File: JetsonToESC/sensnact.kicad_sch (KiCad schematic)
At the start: 8 parts, among them U2 DS18B20

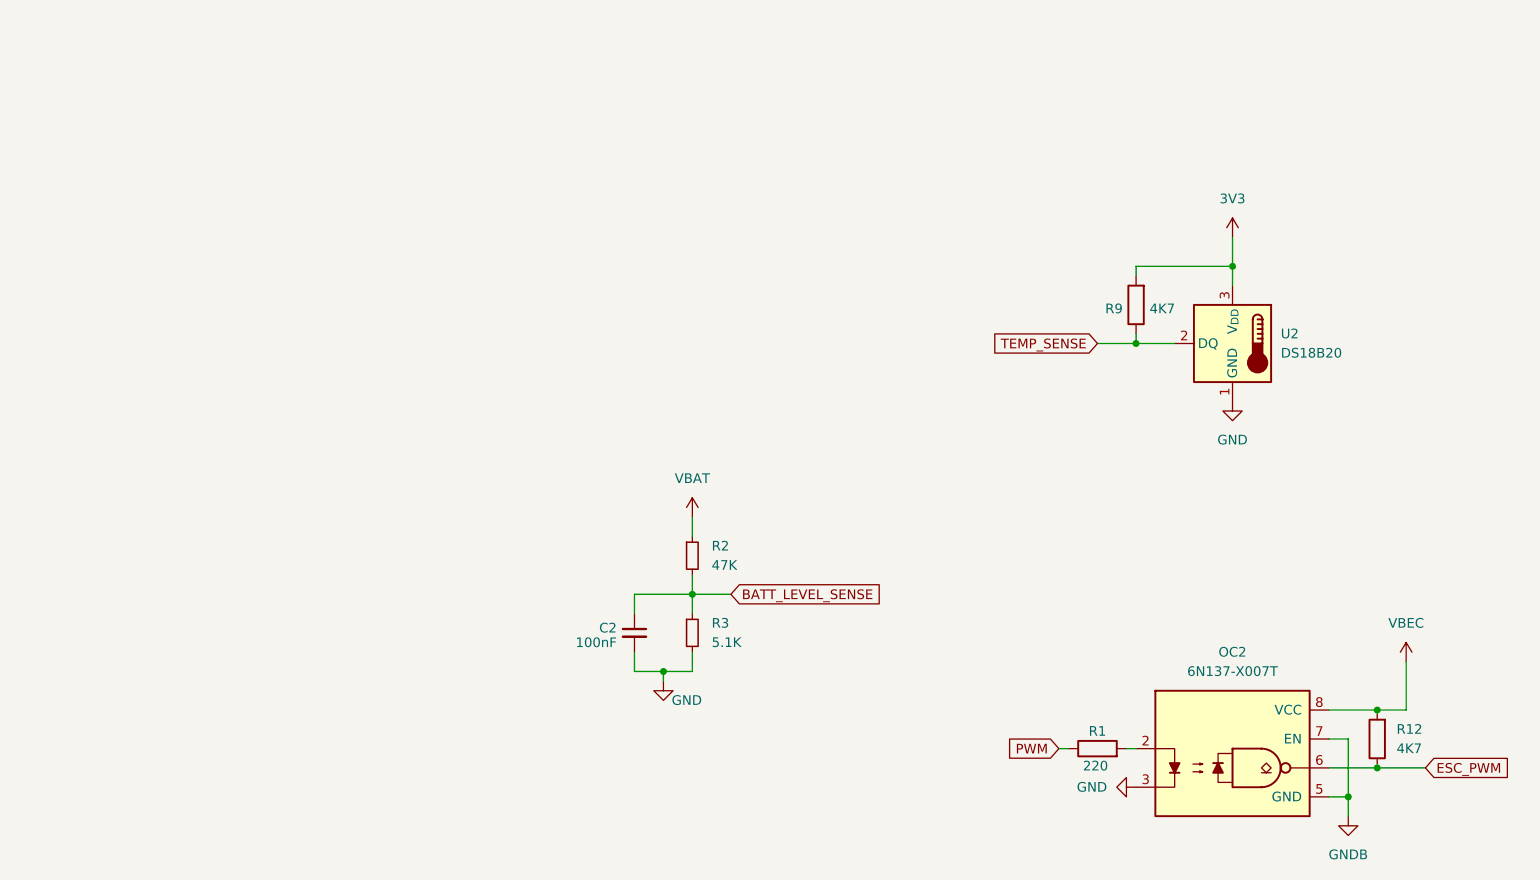
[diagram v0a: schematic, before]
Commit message: Start On this Branch
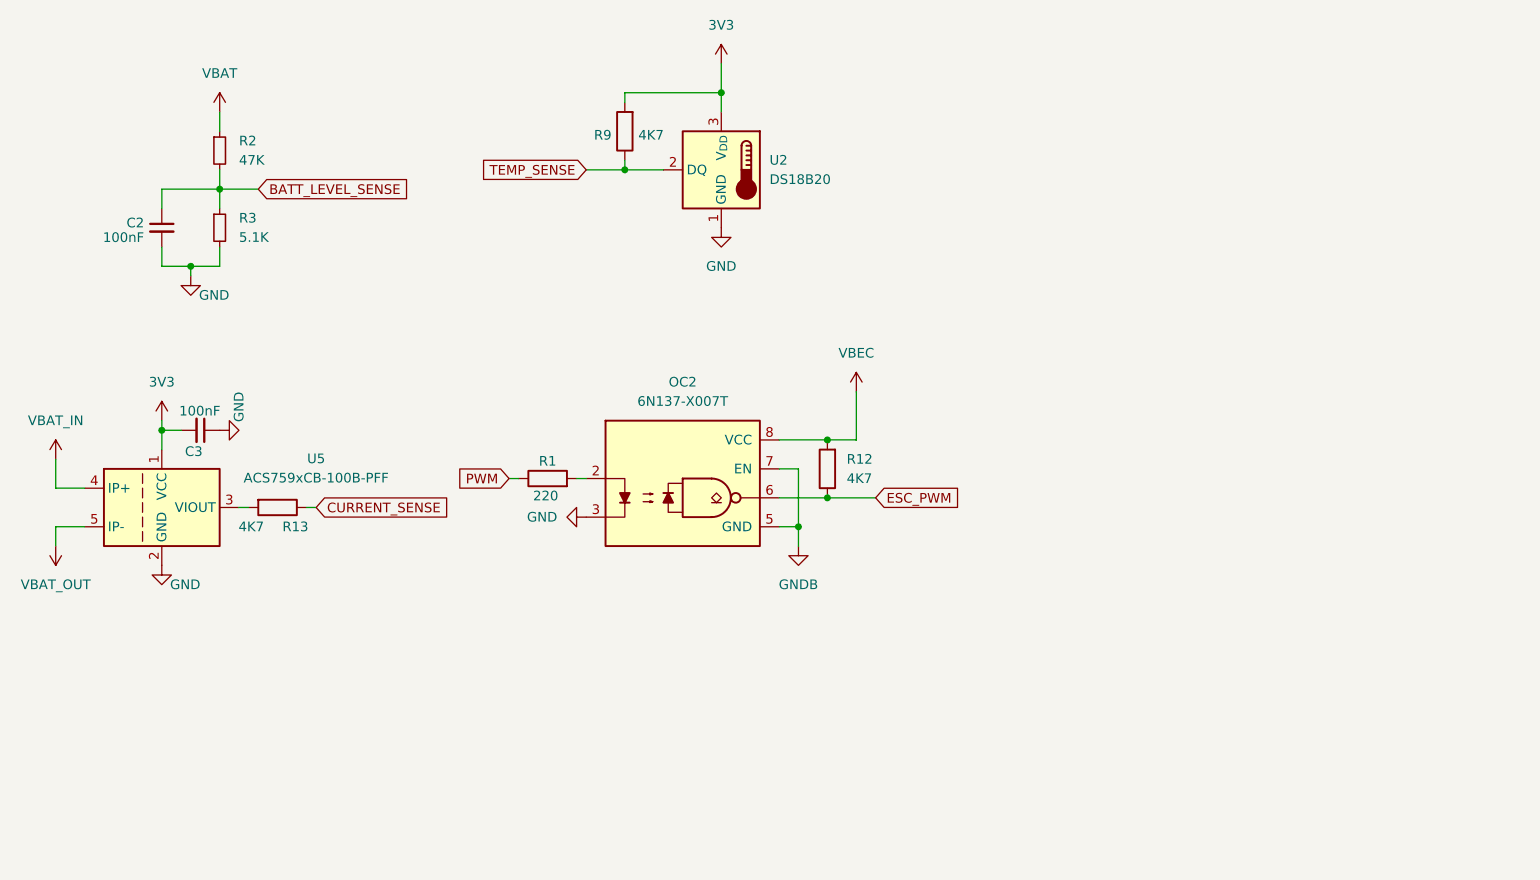
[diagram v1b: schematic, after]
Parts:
- added C3: 100nF, Capacitor_SMD:C_0805_2012Metric_Pad1.18x1.45mm_HandSolder, symbol Device:C_Small
- added R13: 4K7, Resistor_SMD:R_0603_1608Metric, symbol Device:R
- added U5: ACS759xCB-100B-PFF, Sensor_Current:Allegro_CB_PFF, symbol Sensor_Current:ACS759xCB-100B-PFF
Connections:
- net 3V3: now also C3.2, U5.1 (VCC)
- net GND: now also C3.1, U5.2 (GND)
- new net: R13.2, U5.3 (VIOUT)
- new net CURRENT_SENSE: R13.1
- new net VBAT_IN: U5.4 (IP+)
- new net VBAT_OUT: U5.5 (IP-)
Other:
- moved on the sheet: C2, OC2, R1, R12, R2, R3, R9, U2

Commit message: Work on current sense and io expansion branch
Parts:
- C2: footprint Capacitor_SMD:C_0805_2012Metric_Pad1.18x1.45mm_HandSolder -> Capacitor_SMD:C_0603_1608Metric
- R2, R3: footprint Resistor_SMD:R_0805_2012Metric_Pad1.20x1.40mm_HandSolder -> Resistor_SMD:R_0603_1608Metric
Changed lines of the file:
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@@
 			)
 		)
-		(property "Footprint" "Resistor_SMD:R_0805_2012Metric_Pad1.20x1.40mm_HandSolder"
+		(property "Footprint" "Resistor_SMD:R_0603_1608Metric"
 			(at 55.88 46.99 0)
 			(effects
@@
 			)
 		)
-		(property "Footprint" "Resistor_SMD:R_0805_2012Metric_Pad1.20x1.40mm_HandSolder"
+		(property "Footprint" "Resistor_SMD:R_0603_1608Metric"
 			(at 55.88 36.83 0)
 			(effects
@@
 			)
 		)
-		(property "Footprint" "Capacitor_SMD:C_0805_2012Metric_Pad1.18x1.45mm_HandSolder"
+		(property "Footprint" "Capacitor_SMD:C_0603_1608Metric"
 			(at 48.26 46.99 0)
 			(effects
